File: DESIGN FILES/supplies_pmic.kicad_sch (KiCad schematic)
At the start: 0 parts

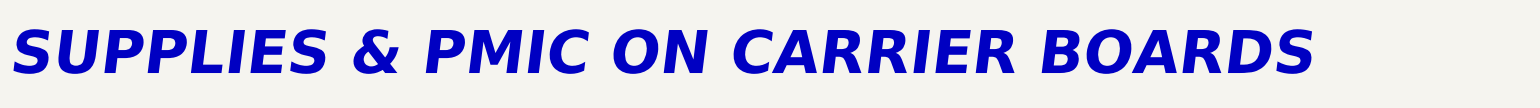
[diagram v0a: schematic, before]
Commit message: updates
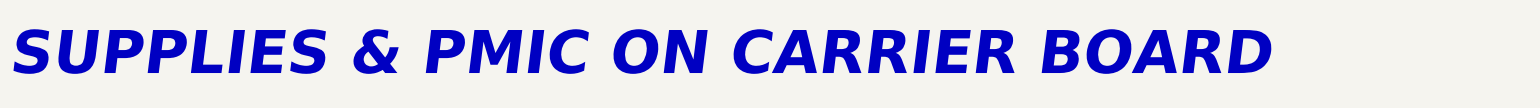
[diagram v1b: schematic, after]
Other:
- note added: "SUPPLIES & PMIC ON CARRIER BOARD"
- note removed: "SUPPLIES & PMIC ON CARRIER BOARDS"
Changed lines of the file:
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@@
     (company "Joël Ucedo")
   )
-  (text "SUPPLIES & PMIC ON CARRIER BOARDS" (at 60.96 147.32 0)
+  (text "SUPPLIES & PMIC ON CARRIER BOARD" (at 60.96 147.32 0)
     (effects (font (size 10 10) (thickness 2) bold italic) (justify left bottom))
   )
